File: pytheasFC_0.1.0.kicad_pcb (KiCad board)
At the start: 4 copper layers, 26.5 x 70.5 mm, 74 parts, among them IC1 BMP390, IC2 ATSAMD21G18A-MFT, IC3 MIC24054YJL-TR, IC4 TLV1117LV33DCYR, J10 Conn_01x02, J13 Conn_01x02, J14 Conn_01x02, J15 Conn_01x02, J4 Conn_02x03, J5 Conn_01x05, J6 Conn_01x05, J7 Conn_01x05, J8 Conn_01x02, J9 Conn_01x02, U2 USBLC6-2SC6, Y1 32.768kHz

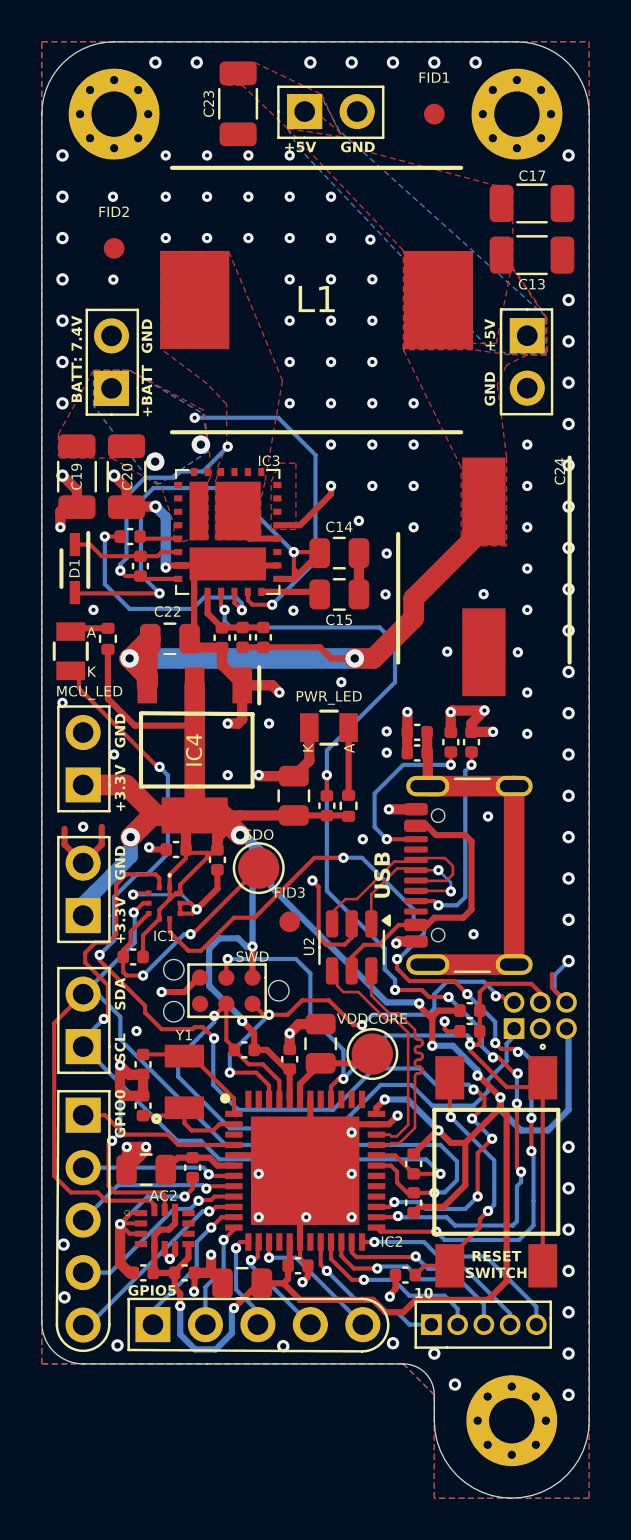
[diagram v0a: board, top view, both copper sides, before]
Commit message: Update Mounting Hole Positions
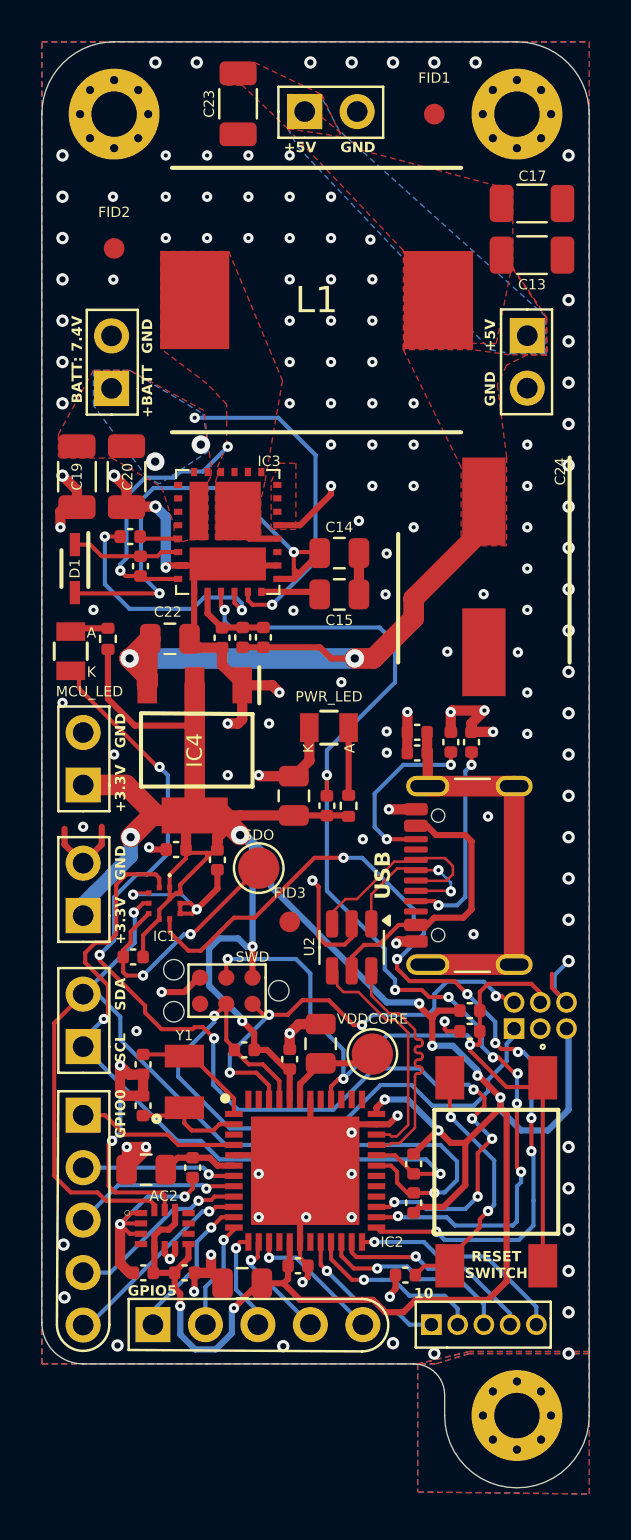
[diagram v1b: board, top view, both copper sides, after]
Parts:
- moved H1 0.35 mm to (221.0, 103.0)
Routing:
- net GND: vias 148 -> 146
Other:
- board size 26.5 x 70.5 mm -> 26.5 x 70 mm
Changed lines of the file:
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@@
 	(footprint "MountingHole:MountingHole_2.2mm_M2_Pad_Via"
 		(layer "F.Cu")
-		(at 220.75 103.25)
+		(at 221 103)
 		(descr "Mounting Hole 2.2mm, M2")
 		(tags "mounting hole 2.2mm m2")
@@
 		(layer "Edge.Cuts")
 	)
-	(gr_line
-		(start 217 103.25)
-		(end 217 102)
+	(gr_arc
+		(start 216 100.5)
+		(mid 217.06066 100.93934)
+		(end 217.5 102)
 		(stroke
 			(width 0.05)
-			(type solid)
+			(type default)
 		)
 		(layer "Edge.Cuts")
 	)
 	(gr_line
-		(start 206 100.5)
-		(end 215.5 100.500001)
+		(start 206 100.499999)
+		(end 216 100.5)
 		(stroke
 			(width 0.05)
@@
 		(layer "Edge.Cuts")
 	)
+	(gr_arc
+		(start 224.5 103)
+		(mid 221 106.5)
+		(end 217.5 103)
+		(stroke
+			(width 0.05)
+			(type solid)
+		)
+		(layer "Edge.Cuts")
+	)
 	(gr_line
 		(start 198 98.5)
@@
 		(layer "Edge.Cuts")
 	)
-	(gr_arc
-		(start 224.5 103.25)
-		(mid 220.75 107)
-		(end 217 103.25)
+	(gr_line
+		(start 217.5 103)
+		(end 217.5 102)
 		(stroke
 			(width 0.05)
-			(type solid)
+			(type default)
 		)
 		(layer "Edge.Cuts")
@@
 	)
 	(gr_line
-		(start 224.5 98.5)
-		(end 224.5 103.25)
-		(stroke
-			(width 0.05)
-			(type solid)
-		)
-		(layer "Edge.Cuts")
-	)
-	(gr_arc
-		(start 215.5 100.5)
-		(mid 216.56066 100.93934)
-		(end 217 102)
-		(stroke
-			(width 0.05)
-			(type solid)
-		)
-		(layer "Edge.Cuts")
-	)
-	(gr_line
 		(start 206 100.5)
 		(end 200 100.5)
@@
 	)
 	(gr_line
-		(start 224.5 98.5)
+		(start 224.5 103)
 		(end 224.5 40)
 		(stroke
@@
 	)
 	(via
-		(at 223.5 102)
-		(size 0.6)
-		(drill 0.3)
-		(layers "F.Cu" "B.Cu")
-		(remove_unused_layers yes)
-		(keep_end_layers yes)
-		(free yes)
-		(zone_layer_connections "In1.Cu" "In2.Cu")
-		(net 1)
-	)
-	(via
 		(at 201.787561 86.052361)
 		(size 0.5)
@@
 	)
 	(via
-		(at 218 101.5)
-		(size 0.6)
-		(drill 0.3)
-		(layers "F.Cu" "B.Cu")
-		(remove_unused_layers yes)
-		(keep_end_layers yes)
-		(free yes)
-		(zone_layer_connections "In1.Cu" "In2.Cu")
-		(net 1)
-	)
-	(via
 		(at 202.584849 84.388802)
 		(size 0.5)
@@
 		(polygon
 			(pts
-				(xy 198 36.5) (xy 224.5 36.5) (xy 224.5 107) (xy 217 107) (xy 217 102) (xy 215.5 100.5) (xy 198 100.5)
+				(xy 198 36.5) (xy 224.5 36.5) (xy 224.5 100) (xy 218.7 100) (xy 217.06066 100.5) (xy 215.5 100.5)
+				(xy 198 100.5)
+			)
+		)
+	)
+	(zone
+		(net 1)
+		(net_name "GND")
+		(layers "F.Cu" "B.Cu" "In1.Cu" "In2.Cu")
+		(hatch edge 0.5)
+		(priority 8)
+		(connect_pads
+			(clearance 0.25)
+		)
+		(min_thickness 0.25)
+		(filled_areas_thickness no)
+		(fill yes
+			(thermal_gap 0.5)
+			(thermal_bridge_width 0.5)
+		)
+		(polygon
+			(pts
+				(xy 216.2 100.5) (xy 216.2 106.7) (xy 224.5 106.8) (xy 224.5 99.9) (xy 218.7 99.9)
 			)
 		)
